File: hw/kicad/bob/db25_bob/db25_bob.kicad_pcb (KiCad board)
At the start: 2 copper layers, 55 parts, among them J1 DB25, J2 DB25, P1 DIL8, P2 DIL8, P3 DIL6, P4 DIL8, P5 DIL8, P6 DIL8, U1 ADuM1201WT, U2 ADuM1201WT, U3 ADuM1201WT, U4 ADuM1201WT, U5 ADuM1201WT, U6 ADuM1201WT, U7 ADuM1201WT, U8 ADuM1201WT

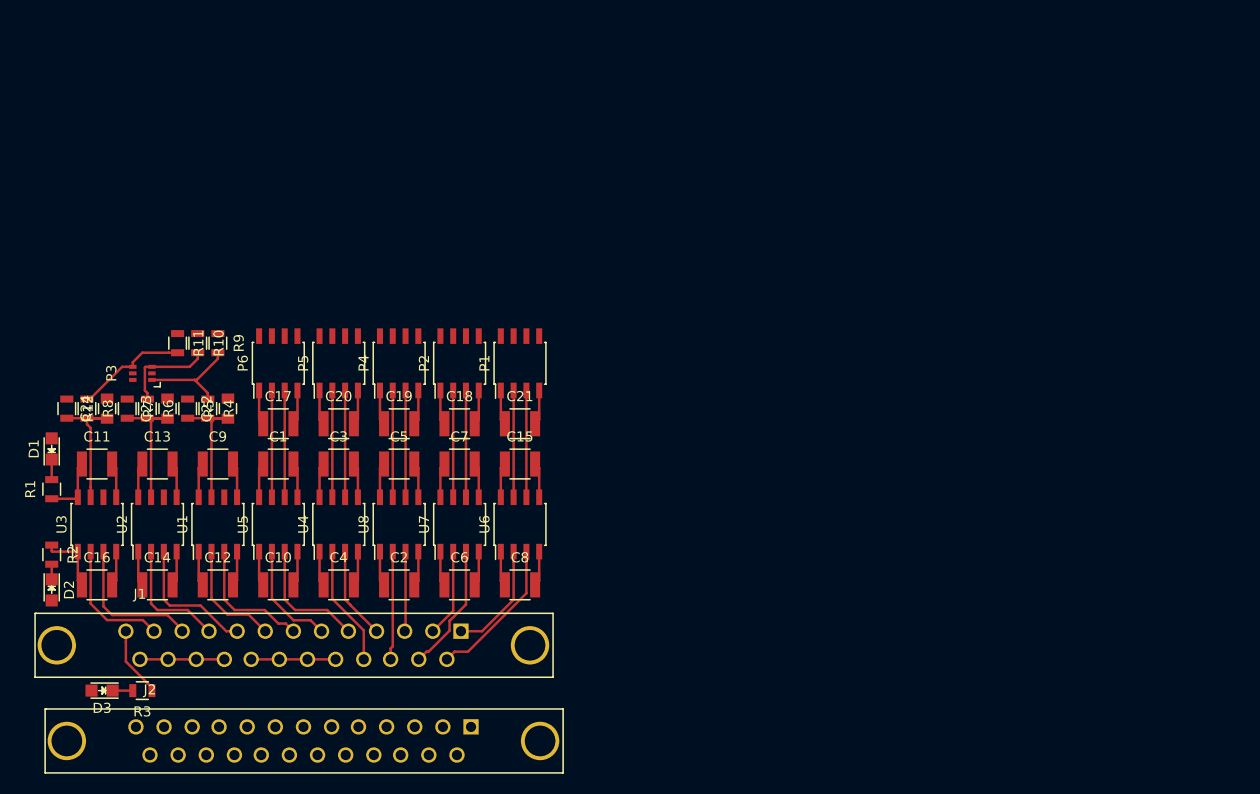
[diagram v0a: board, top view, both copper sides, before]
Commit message: Latest changes.
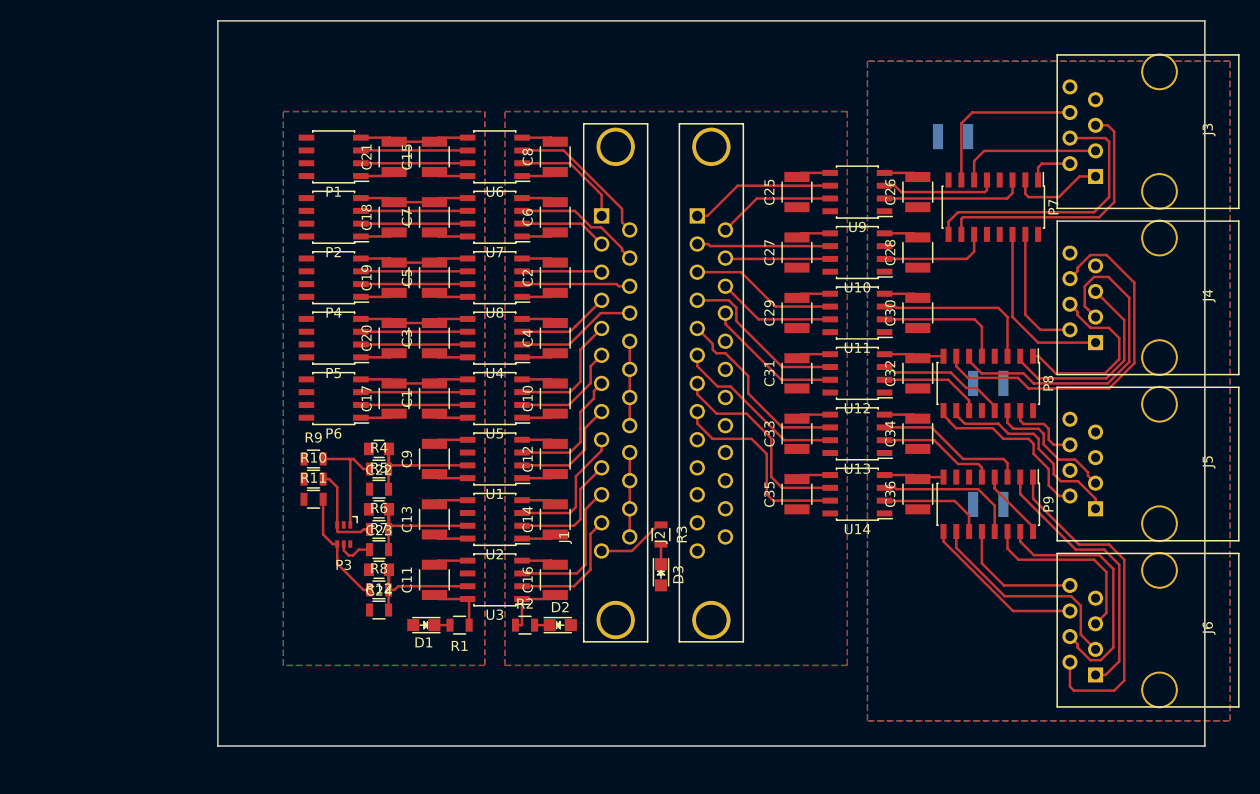
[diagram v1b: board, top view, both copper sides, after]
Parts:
- added C25: C, Capacitors_SMD:C_1210, F.Cu at (199.5, 87.0)
- added C26: C, Capacitors_SMD:C_1210, F.Cu at (211.5, 87.0)
- added C27: C, Capacitors_SMD:C_1210, F.Cu at (199.5, 93.0)
- added C28: C, Capacitors_SMD:C_1210, F.Cu at (211.5, 93.0)
- added C29: C, Capacitors_SMD:C_1210, F.Cu at (199.5, 99.0)
- added C30: C, Capacitors_SMD:C_1210, F.Cu at (211.5, 99.0)
- added C31: C, Capacitors_SMD:C_1210, F.Cu at (199.5, 105.0)
- added C32: C, Capacitors_SMD:C_1210, F.Cu at (211.5, 105.0)
- added C33: C, Capacitors_SMD:C_1210, F.Cu at (199.5, 111.0)
- added C34: C, Capacitors_SMD:C_1210, F.Cu at (211.5, 111.0)
- added C35: C, Capacitors_SMD:C_1210, F.Cu at (199.5, 117.0)
- added C36: C, Capacitors_SMD:C_1210, F.Cu at (211.5, 117.0)
- added C37: C, Capacitors_SMD:C_1210, B.Cu at (215.0, 81.5)
- added C38: C, Capacitors_SMD:C_1210, B.Cu at (218.5, 106.0)
- added C39: C, Capacitors_SMD:C_1210, B.Cu at (218.5, 118.0)
- added J3: RJ45, Connect:RJ45_8, F.Cu at (235.5, 81.0)
- added J4: RJ45, Connect:RJ45_8, F.Cu at (235.5, 97.5)
- added J5: RJ45, Connect:RJ45_8, F.Cu at (235.5, 114.0)
- added J6: RJ45, Connect:RJ45_8, F.Cu at (235.5, 130.5)
- added P7: DIL16, Housings_SOIC:SOIC-16_3.9x9.9mm_Pitch1.27mm, F.Cu at (219.0, 88.5)
- added P8: DIL16, Housings_SOIC:SOIC-16_3.9x9.9mm_Pitch1.27mm, F.Cu at (218.5, 106.0)
- added P9: DIL16, Housings_SOIC:SOIC-16_3.9x9.9mm_Pitch1.27mm, F.Cu at (218.5, 118.0)
- added U10: ADuM1200CR, Housings_SOIC:SOIC-8_3.9x4.9mm_Pitch1.27mm, F.Cu at (205.5, 93.0)
- added U11: ADuM1200CR, Housings_SOIC:SOIC-8_3.9x4.9mm_Pitch1.27mm, F.Cu at (205.5, 99.0)
- added U12: ADuM1200CR, Housings_SOIC:SOIC-8_3.9x4.9mm_Pitch1.27mm, F.Cu at (205.5, 105.0)
- added U13: ADuM1200CR, Housings_SOIC:SOIC-8_3.9x4.9mm_Pitch1.27mm, F.Cu at (205.5, 111.0)
- added U14: ADuM1200CR, Housings_SOIC:SOIC-8_3.9x4.9mm_Pitch1.27mm, F.Cu at (205.5, 117.0)
- added U9: ADuM1200CR, Housings_SOIC:SOIC-8_3.9x4.9mm_Pitch1.27mm, F.Cu at (205.5, 87.0)
- moved D3 56.7 mm to (186.0, 125.0), turned to 270 degrees
- moved J2 53.9 mm to (191.0, 106.0), turned to 90 degrees
- moved R3 53.8 mm to (186.0, 121.0), turned to 270 degrees
- moved D2 50.6 mm to (176.0, 130.0), turned to 0 degrees
- moved R2 47.5 mm to (172.5, 130.0), turned to 0 degrees
- moved C16 45.5 mm to (175.5, 125.5), turned to 90 degrees
- moved R1 42.7 mm to (166.0, 130.0), turned to 180 degrees
- moved C8 42.6 mm to (175.5, 83.5), turned to 90 degrees
- moved J1 41.2 mm to (181.5, 106.0), turned to 90 degrees
- moved D1 40.9 mm to (162.5, 130.0), turned to 180 degrees
- moved C14 40.0 mm to (175.5, 119.5), turned to 90 degrees
- moved U3 39.9 mm to (169.5, 125.5), turned to 180 degrees
- moved C6 37.7 mm to (175.5, 89.5), turned to 90 degrees
- moved R12 36.9 mm to (158.0, 128.5), turned to 0 degrees
- moved U6 36.6 mm to (169.5, 83.5), turned to 180 degrees
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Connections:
- net GNDA renamed EN-
- J2 pad 1: Net-(J2-Pad1) -> ENC0BO
- J2 pad 14: Net-(J2-Pad14) -> ENC0AO
- J2 pad 15: Net-(J2-Pad15) -> ENC0ZO
- J2 pad 16: Net-(J2-Pad16) -> ENC1BO
- J2 pad 17: Net-(J2-Pad17) -> ENC2AO
- J2 pad 18: Net-(J2-Pad18) -> GND
- J2 pad 19: Net-(J2-Pad19) -> GND
- J2 pad 2: Net-(J2-Pad2) -> ENC1AO
- J2 pad 20: Net-(J2-Pad20) -> GND
- J2 pad 21: Net-(J2-Pad21) -> GND
- J2 pad 22: Net-(J2-Pad22) -> +5V
- J2 pad 23: Net-(J2-Pad23) -> +5V
- J2 pad 24: Net-(J2-Pad24) -> +5V
- J2 pad 25: Net-(J2-Pad25) -> +5V
- J2 pad 3: Net-(J2-Pad3) -> ENC1ZO
- J2 pad 4: Net-(J2-Pad4) -> ENC2BO
- J2 pad 5: Net-(J2-Pad5) -> ENC3AO
- J2 pad 6: Net-(J2-Pad6) -> ENC2ZO
- J2 pad 7: Net-(J2-Pad7) -> ENC3ZO
- J2 pad 8: Net-(J2-Pad8) -> ENC3BO
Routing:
- net EN-: track 45.1 -> 104.0 mm
- net ENC1B-: track 0.00 -> 37.3 mm
- net ENC3A-: track 0.00 -> 34.1 mm
- net ENC1B+: track 0.00 -> 33.7 mm
- net ENC0Z-: track 0.00 -> 27.8 mm
- net ENC3A+: track 0.00 -> 26.9 mm
- net ENC0Z+: track 0.00 -> 26.5 mm
- net ENC3Z-: track 0.00 -> 25.2 mm
- net ENC3B+: track 0.00 -> 21.3 mm
- net GND: track 36.1 -> 56.9 mm
- net ENC3ZO: track 0.00 -> 20.4 mm
- net ENC1Z+: track 0.00 -> 20.3 mm
- net ENC3BO: track 0.00 -> 19.9 mm
- net ENC2A+: track 0.00 -> 19.9 mm
- net ENC3AO: track 0.00 -> 18.6 mm
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- added copper zone on F.Cu, net +5V
- added copper zone on F.Cu, net +5VA
- added copper zone on B.Cu, net EN-
- added copper zone on B.Cu, net GND
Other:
- board outline added: 98 x 72 mm
